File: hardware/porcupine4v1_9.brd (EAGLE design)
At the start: 24.4 x 27.4 mm, 28 parts, among them X1 PROGCON

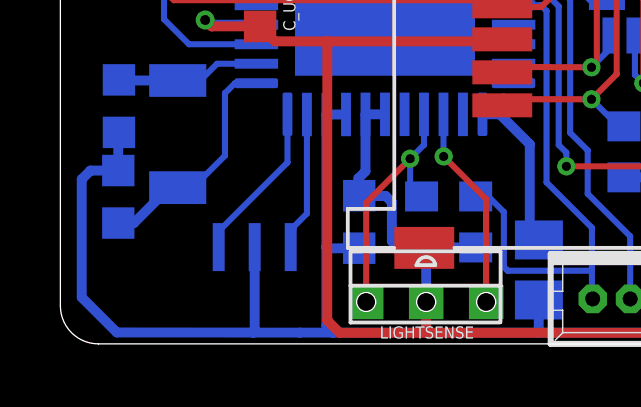
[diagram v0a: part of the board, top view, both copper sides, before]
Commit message: v4.1.9: added farnell order numbers
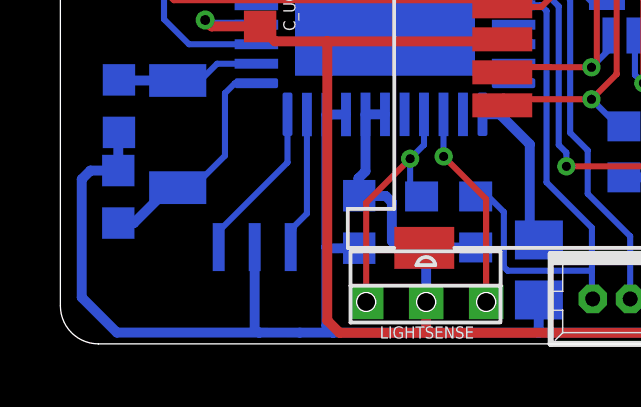
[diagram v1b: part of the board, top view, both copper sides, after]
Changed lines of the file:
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@@
 <attribute name="VALUE" x="22.8092" y="14.6304" size="1.016" layer="27" rot="R180"/>
 <attribute name="NAME" x="22.0726" y="16.2306" size="0.4064" layer="25" rot="R180"/>
-</element>
-<element name="LIGHTSENSE" library="HedgehogLib" package="TSL" value="TSL250" x="12.192" y="1.397" rot="R180"/>
+<attribute name="OC_FARNELL" value="1686452" x="24.0792" y="3.2004" size="1.778" layer="27" rot="R180" display="off"/>
+</element>
+<element name="LIGHTSENSE" library="HedgehogLib" package="TSL" value="TSL250" x="12.192" y="1.397" rot="R180">
+<attribute name="OC_FARNELL" value="1182346" x="12.192" y="1.397" size="1.778" layer="27" rot="R180" display="off"/>
+</element>
 <element name="USB_CON" library="HedgehogLib" package="248601" value="USBCON" x="18.7216" y="22.9344" smashed="yes" rot="R270">
 <attribute name="NAME" x="17.4262" y="22.0962" size="0.4064" layer="25"/>
 <attribute name="VALUE" x="11.7366" y="27.3794" size="1.27" layer="27" rot="R270"/>
+<attribute name="OC_FARNELL" value="2112367" x="18.7216" y="22.9344" size="1.778" layer="27" rot="R270" display="off"/>
 </element>
 <element name="C_PWR_VUSB" library="rcl" package="C0603K" value="1u" x="3.7024" y="17.4952" smashed="yes">
@@
 <attribute name="NAME" x="22.9616" y="9.271" size="0.4064" layer="26" rot="MR0"/>
 <attribute name="VALUE" x="22.352" y="8.9662" size="0.4064" layer="28" rot="MR0"/>
+<attribute name="OC_FARNELL" value="1853935" x="20.32" y="11.3792" size="1.778" layer="28" rot="MR0" display="off"/>
 </element>
 <element name="C_ADX_VDD" library="rcl" package="C0603K" value="0.1u" x="19.2024" y="14.0716" smashed="yes" rot="MR180">
@@
 <attribute name="NAME" x="13.2218" y="8.4108" size="0.4064" layer="26" rot="MR0"/>
 <attribute name="VALUE" x="16.3454" y="15.838" size="1.27" layer="28" rot="MR270"/>
+<attribute name="OC_FARNELL" value="1706311" x="10.8204" y="11.938" size="1.778" layer="28" rot="MR270" display="off"/>
 </element>
 <element name="C2_32KHZ" library="rcl" package="C0603K" value="22p" x="1.9304" y="4.9022" smashed="yes" rot="MR90">
@@
 </element>
 <element name="32KHZ_CRYSTAL" library="HedgehogLib" package="SMD_CRYSTAL" value="SMD_CRYSTAL" x="3.9116" y="6.985" rot="MR90">
-<attribute name="FARNELL" value="2101349" x="3.9116" y="6.985" size="1.778" layer="28" rot="MR90" display="off"/>
+<attribute name="OC_FARNELL" value="2101349" x="3.9116" y="6.985" size="1.778" layer="28" rot="MR90" display="off"/>
 </element>
 <element name="BAT" library="con-molex" package="53048-02" value="53048-02" x="2.667" y="24.3586" smashed="yes" rot="R270">
@@
 </element>
 <element name="12MHZ_RESONATOR" library="HedgehogLib" package="PRQC-C" value="RESONATORPRQC-C" x="6.477" y="3.2258" rot="MR180">
-<attribute name="DIGIKEY" value="http://www.digikey.de/product-detail/de/PRQC12.00CR5010X000/478-6318-1-ND/2506334" x="6.477" y="3.2258" size="1.778" layer="28" rot="MR180" display="off"/>
+<attribute name="OC_DIGIKEY" value="478-6318-1-ND" x="6.477" y="3.2258" size="1.778" layer="28" rot="MR180" display="off"/>
 </element>
 <element name="LDO" library="HedgehogLib" package="SOT-23-5" value="MCP1824" x="7.366" y="23.8252" smashed="yes" rot="MR90">
 <attribute name="NAME" x="7.9248" y="25.4762" size="0.4064" layer="26" rot="MR0"/>
 <attribute name="VALUE" x="4.191" y="21.9202" size="1.27" layer="28" rot="MR90"/>
+<attribute name="OC_FARNELL" value="1578387" x="7.366" y="23.8252" size="1.778" layer="28" rot="MR90" display="off"/>
 </element>
 </elements>
@@
 <wire x1="4.5352" y1="12.3304" x2="6.6576" y2="12.3304" width="0.3302" layer="1"/>
 <wire x1="9.0932" y1="0.3756" x2="7.981" y2="0.3756" width="0.3302" layer="16"/>
-<wire x1="7.981" y1="0.3756" x2="6.425746875" y2="0.376975" width="0.3302" layer="16"/>
-<wire x1="6.425746875" y1="0.376975" x2="1.8796" y2="0.381" width="0.3302" layer="16"/>
+<wire x1="7.981" y1="0.3756" x2="6.628946875" y2="0.376975" width="0.3302" layer="16"/>
 <wire x1="1.9304" y1="5.7772" x2="1.9304" y2="6.8072" width="0.3302" layer="16"/>
 <wire x1="1.9304" y1="6.8072" x2="1.952" y2="7.0498" width="0.3302" layer="16"/>
@@
 <wire x1="1.002" y1="5.7772" x2="0.7112" y2="5.4864" width="0.3302" layer="16"/>
 <wire x1="6.477" y1="3.2258" x2="6.477" y2="0.428228125" width="0.3302" layer="16"/>
-<wire x1="6.477" y1="0.428228125" x2="6.425746875" y2="0.376975" width="0.3302" layer="16"/>
-<wire x1="1.8796" y1="0.381" x2="0.7112" y2="1.5494" width="0.3302" layer="16"/>
+<wire x1="6.477" y1="0.428228125" x2="6.628946875" y2="0.376975" width="0.3302" layer="16"/>
 <wire x1="0.7112" y1="1.5494" x2="0.7112" y2="5.4864" width="0.3302" layer="16"/>
 <wire x1="5.0038" y1="25.9448" x2="11.176" y2="25.9448" width="0.3302" layer="16"/>
@@
 <wire x1="4.2926" y1="24.638" x2="4.0754" y2="24.8666" width="0.3302" layer="16"/>
 <wire x1="4.0754" y1="24.8666" x2="3.683" y2="24.624" width="0.3302" layer="16"/>
+<wire x1="6.628946875" y1="0.376975" x2="1.883625" y2="0.376975" width="0.3302" layer="16"/>
+<wire x1="1.883625" y1="0.376975" x2="0.7112" y2="1.5494" width="0.3302" layer="16"/>
 </signal>
 <signal name="USB_D+@RC5">
